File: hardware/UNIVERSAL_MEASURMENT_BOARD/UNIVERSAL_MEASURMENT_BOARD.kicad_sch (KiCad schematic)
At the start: 0 parts

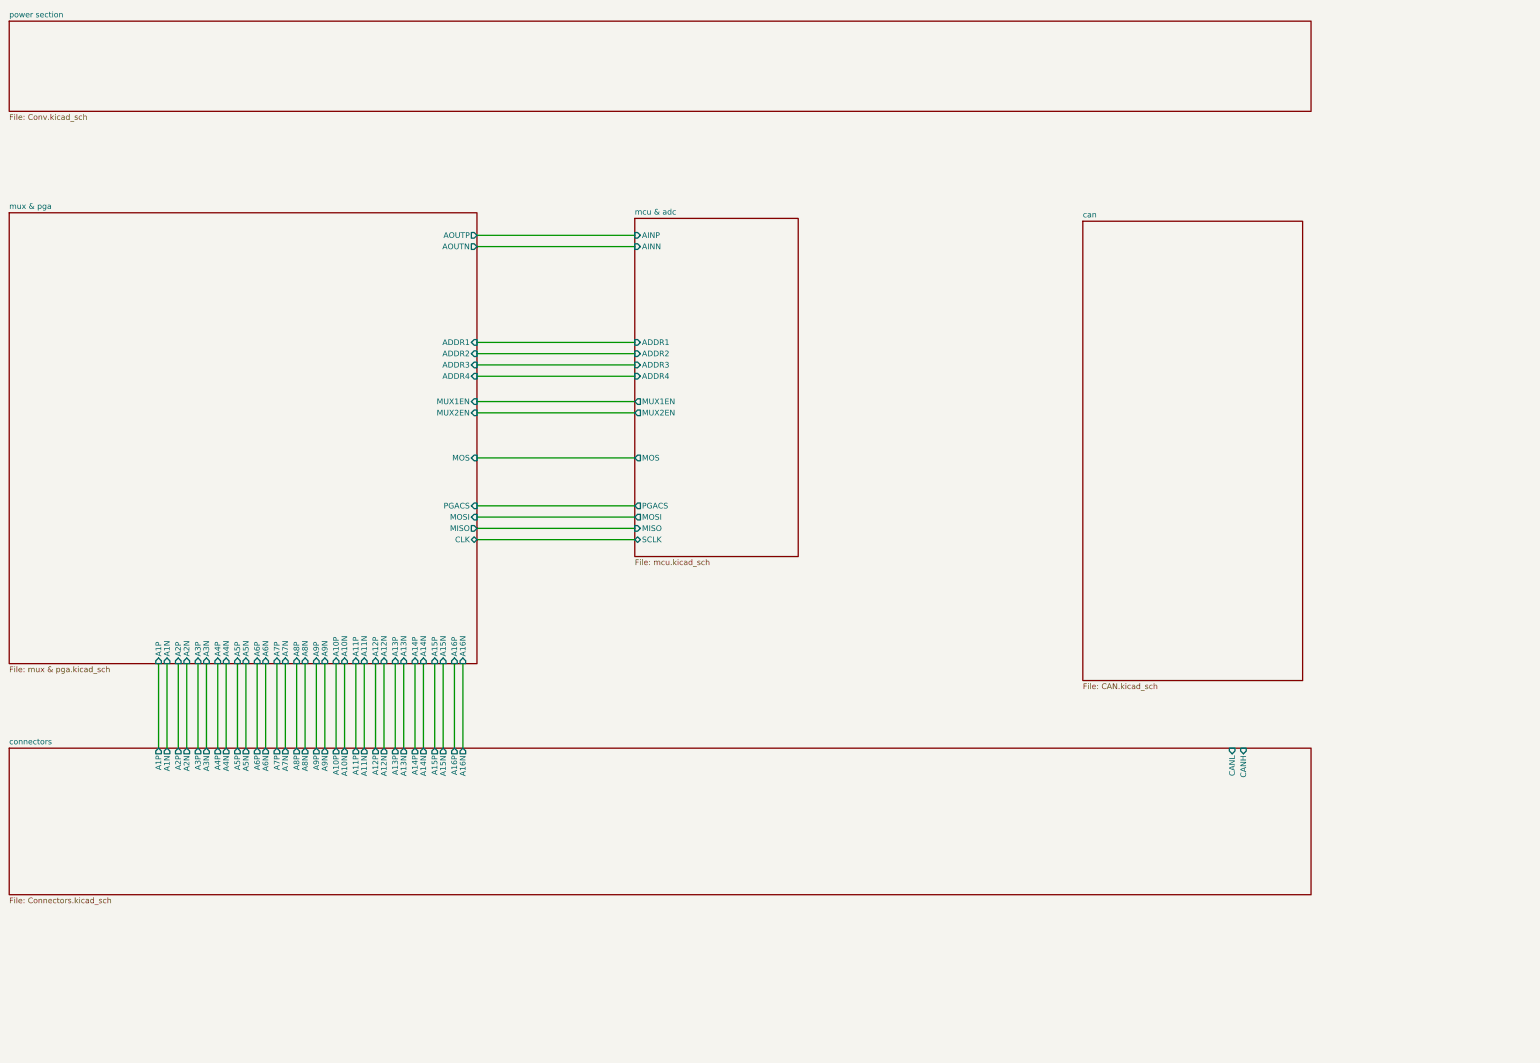
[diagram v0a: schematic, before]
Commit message: continued
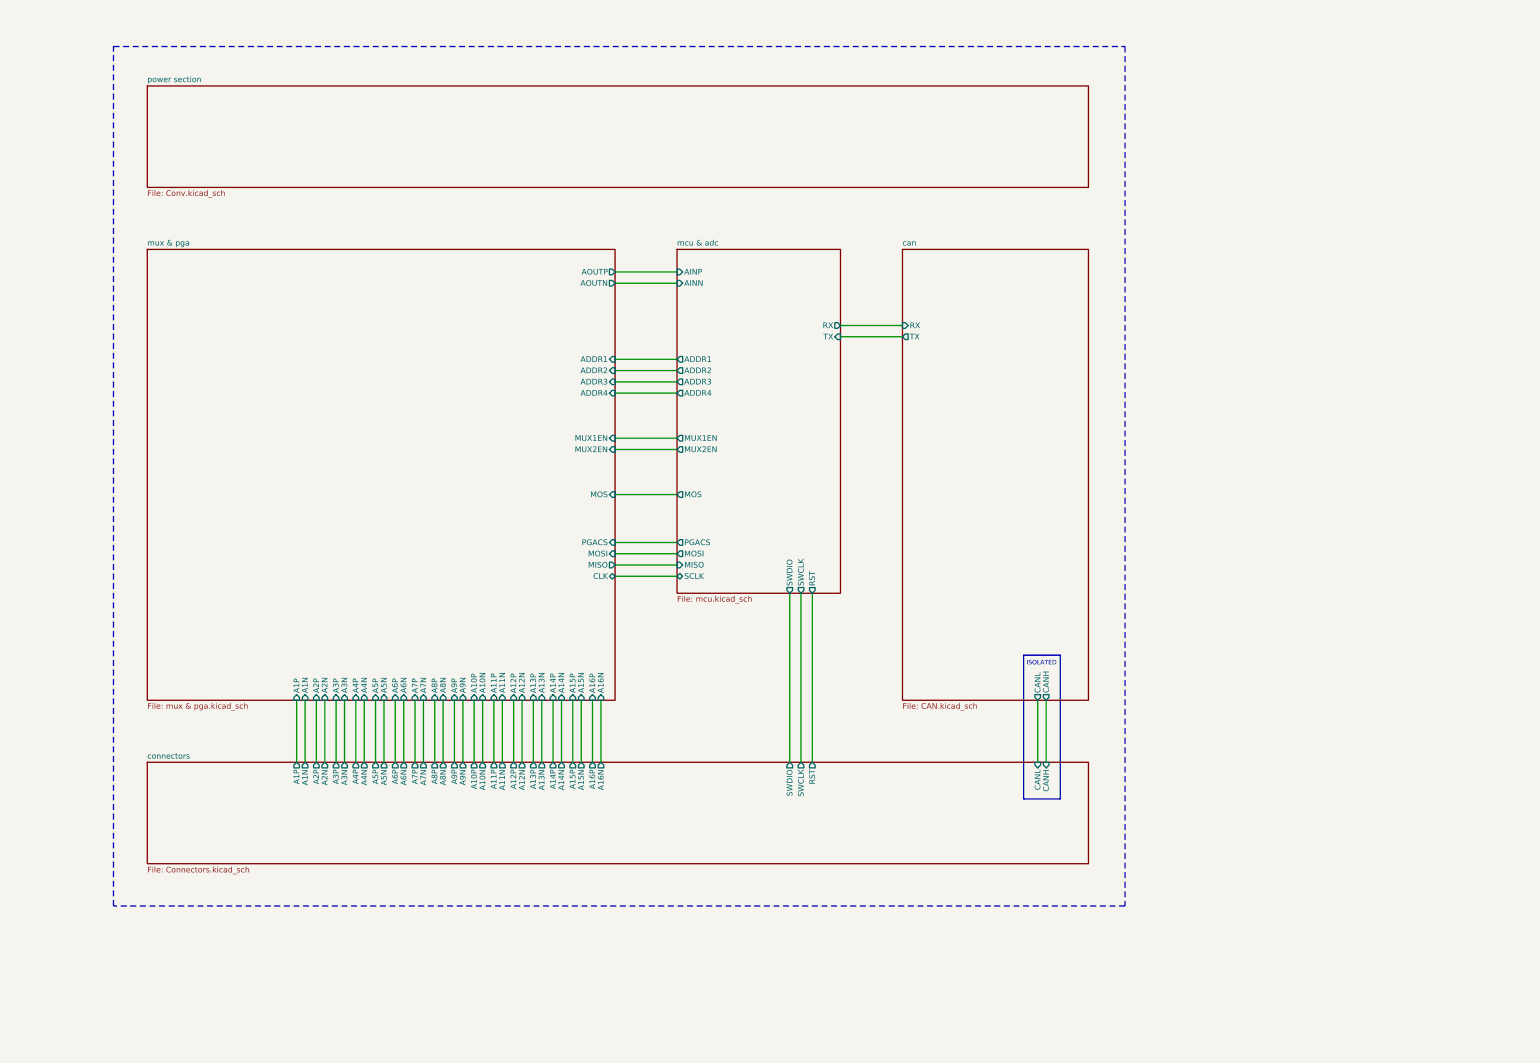
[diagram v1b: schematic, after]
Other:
- sheet can ports: added CANH, CANL, RX, TX; removed none
- sheet connectors ports: added RST, SWCLK, SWDIO; removed none
- sheet mcu & adc ports: added RST, RX, SWCLK, SWDIO, TX; removed none
- note added: "ISOLATED"
- company: (none) -> PUT Motorsport Formula Student team
- title: (none) -> Universal Measurment Board

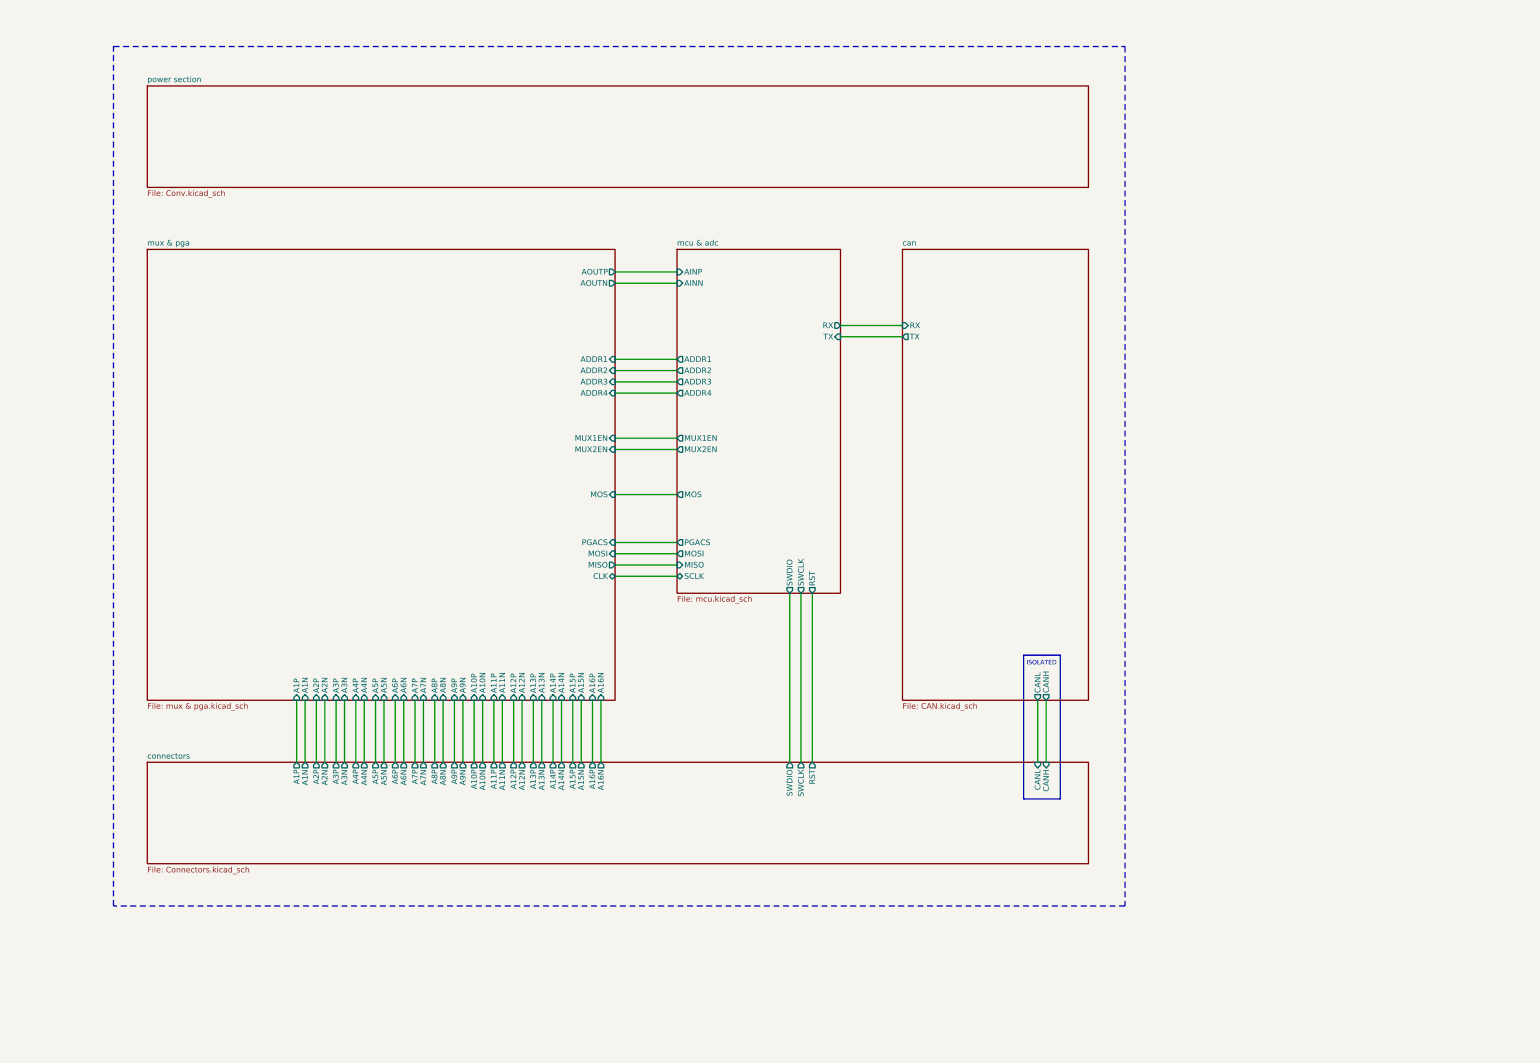
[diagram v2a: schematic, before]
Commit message: final schematic review corrections
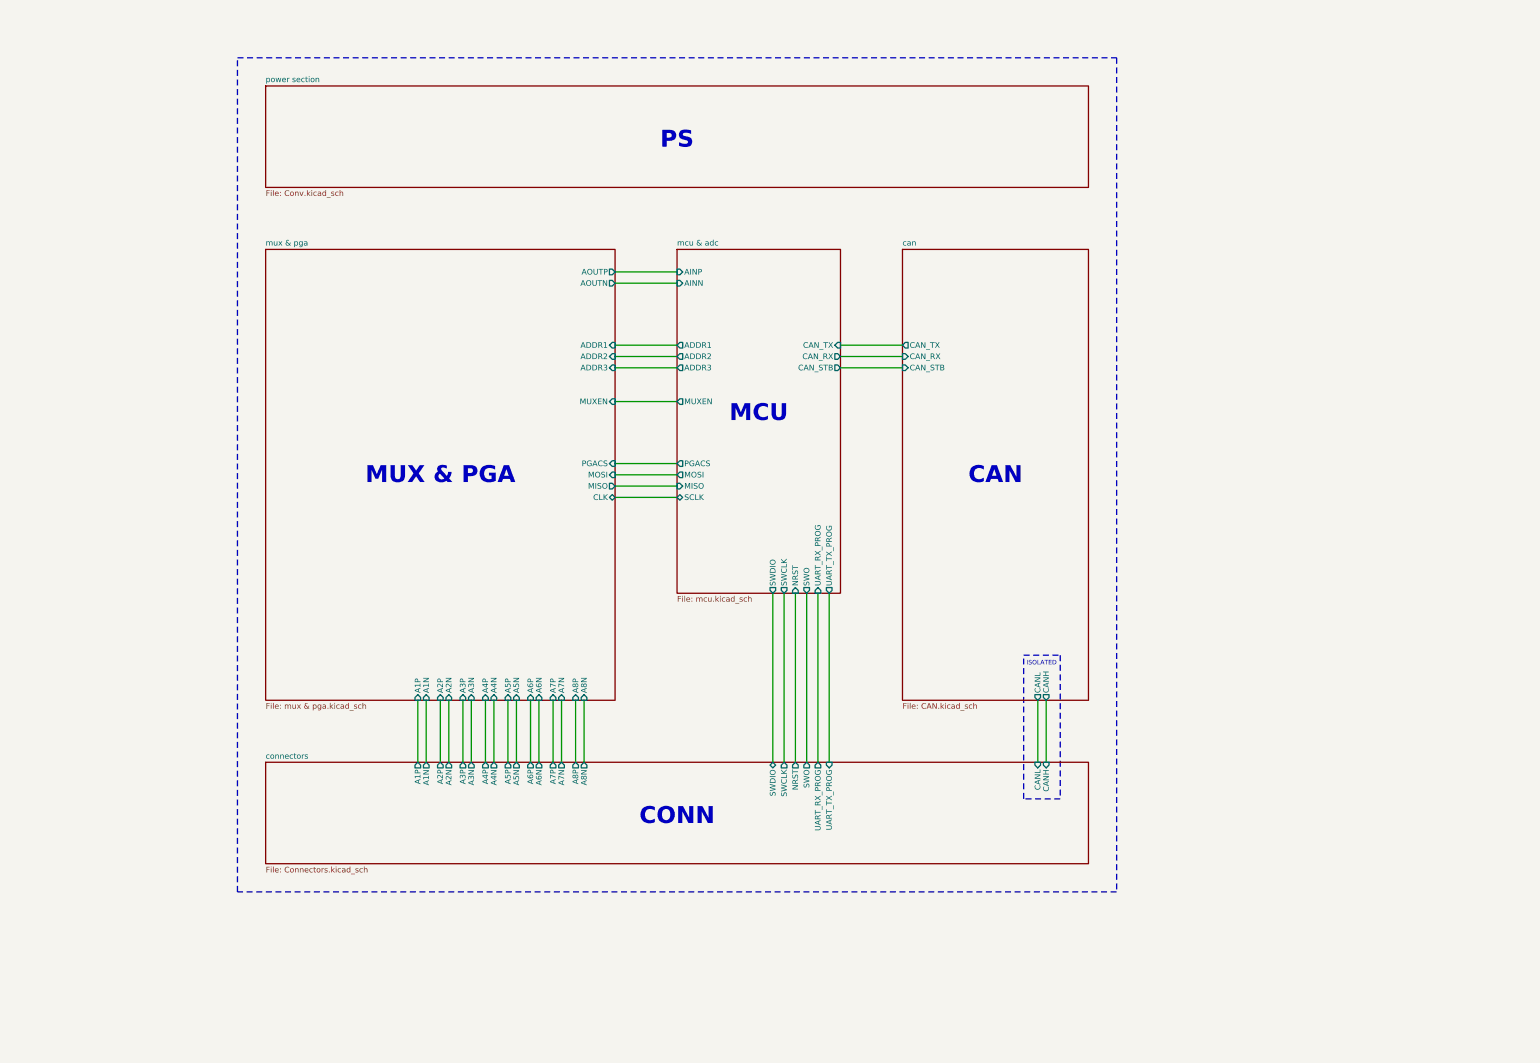
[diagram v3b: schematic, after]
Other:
- sheet can ports: added CAN_RX, CAN_STB, CAN_TX; removed RX, TX
- sheet connectors ports: added NRST, SWO, UART_RX_PROG, UART_TX_PROG; removed A10N, A10P, A11N, A11P, A12N, A12P, A13N, A13P, A14N, A14P, A15N, A15P, A16N, A16P, A9N, A9P, RST
- sheet mcu & adc ports: added CAN_RX, CAN_STB, CAN_TX, MUXEN, NRST, SWO, UART_RX_PROG, UART_TX_PROG; removed ADDR4, MOS, MUX1EN, MUX2EN, RST, RX, TX
- sheet mux & pga ports: added MUXEN; removed A10N, A10P, A11N, A11P, A12N, A12P, A13N, A13P, A14N, A14P, A15N, A15P, A16N, A16P, A9N, A9P, ADDR4, MOS, MUX1EN, MUX2EN
- note added: "CAN"
- note added: "CONN"
- note added: "MCU"
- note added: "MUX & PGA"
- note added: "PS"

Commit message: added footprints
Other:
- company: PUT Motorsport Formula Student team -> PUT Motorsport Formula Student Team
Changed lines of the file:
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@@
 		(title "Universal Measurment Board")
 		(date "2026-02-02")
-		(rev "1.7.14")
-		(company "PUT Motorsport Formula Student team")
+		(rev "1.7.15")
+		(company "PUT Motorsport Formula Student Team")
 		(comment 1 "Designed by Marcin Trzmiel under")
 	)

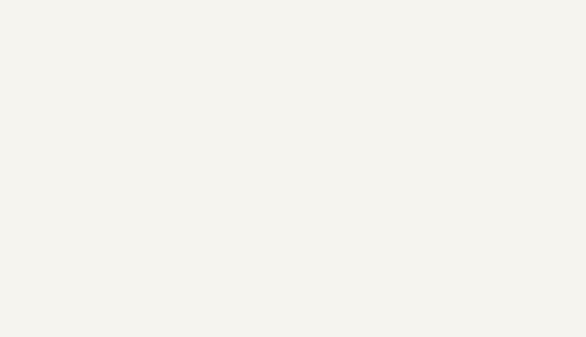
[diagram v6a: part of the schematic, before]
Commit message: clean up project visuals
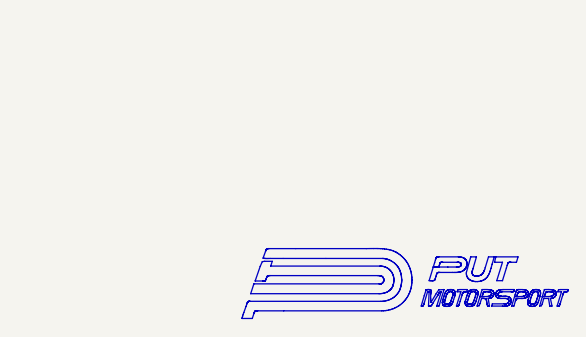
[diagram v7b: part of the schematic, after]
